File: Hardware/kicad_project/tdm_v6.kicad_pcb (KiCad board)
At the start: 4 copper layers, 65 x 100 mm, 139 parts, among them J1 line_in, J2 headphone_out, J3 battery, J4 DebugHeader, Q1 DMG2305UX-13, SW1 spst_4_pin_internal, SW10 spst_4_pin_internal, SW11 spst_4_pin_internal, SW12 spst_4_pin_internal, SW13 spst_4_pin_internal, SW14 spst_4_pin_internal, SW15 spst_4_pin_internal, SW16 spst_4_pin_internal, SW17 spst_4_pin_internal, SW18 spst_4_pin_internal, SW19 spst_4_pin_internal, SW2 spst_4_pin_internal, SW20 spst_4_pin_internal, SW21 spst_4_pin_internal, SW22 spst_4_pin_internal, SW23 spst_4_pin_internal, SW24 spst_4_pin_internal, SW25 spst_4_pin_internal, SW26 spst_4_pin_internal, SW3 spst_4_pin_internal, SW4 spst_4_pin_internal, SW5 spst_4_pin_internal, SW6 spst_4_pin_internal, SW7 spst_4_pin_internal, SW8 spst_4_pin_internal, SW9 spst_4_pin_internal, U2 Pico, U3 TLV320AIC3204, U4 SPWmicrophone, U5 MCP73831T-2ATI_OT

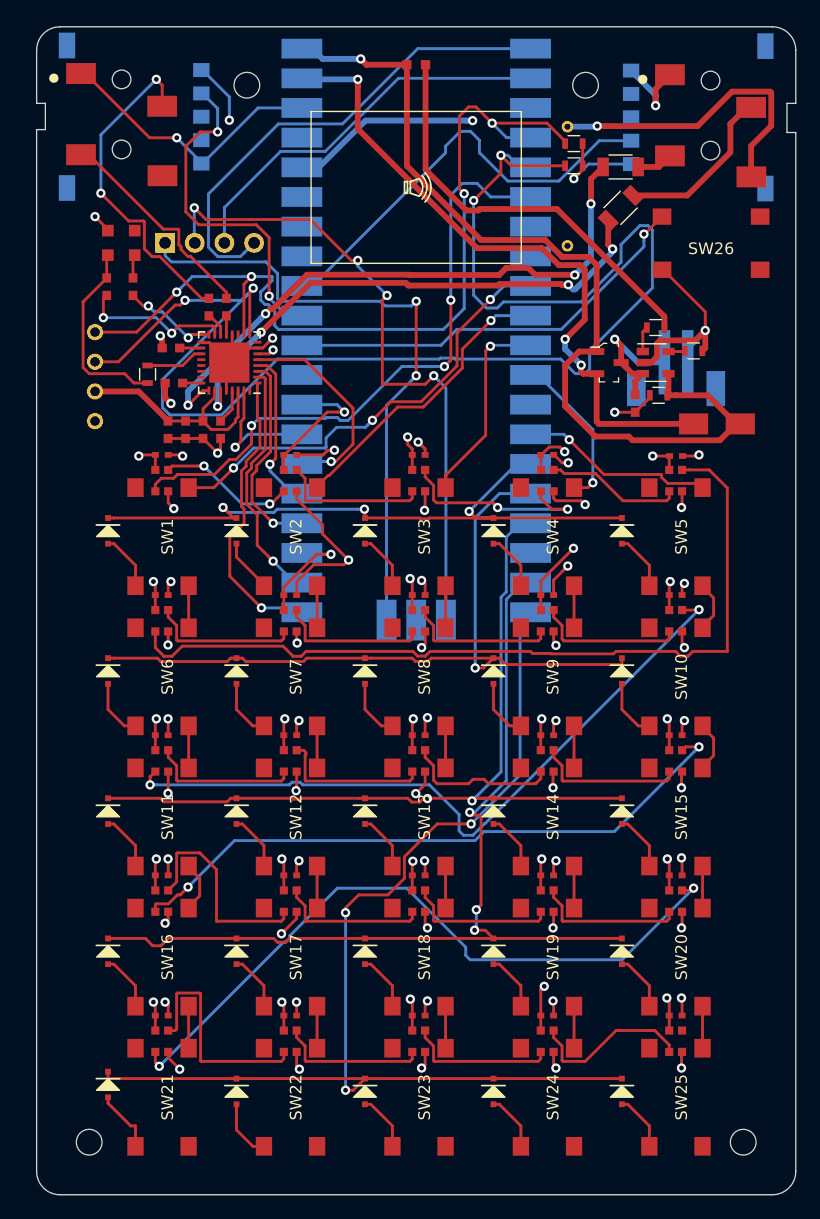
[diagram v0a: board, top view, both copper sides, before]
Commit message: update project with corrected schematic / pcb
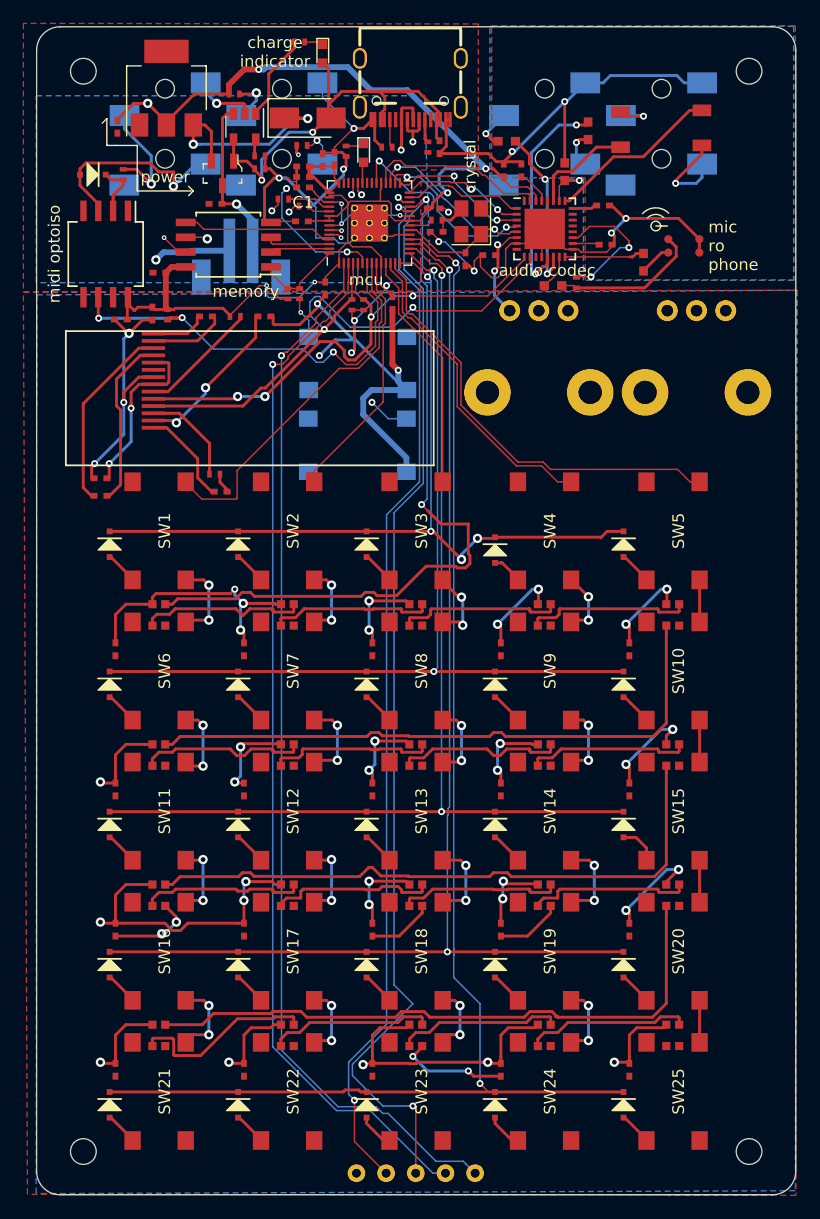
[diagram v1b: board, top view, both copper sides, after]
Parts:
- removed C2, C3, C4, C5: 1u, RandomJunk:C_0402_NoSilk
- removed D1, D2, D3, D4, D5: D, RandomJunk:D_SOD-323F_less_silk
- removed LS1: Speaker, RandomJunk:CMS-181325
- removed OL1: OLED, kbd:OLED_v2
- added C39: .47u, RandomJunk:C_0603_nosilk, F.Cu at (80.5, 40.8)
- added C40: .1uF, RandomJunk:C_0603_nosilk, F.Cu at (78.5, 44.2)
- added C41: 1u, RandomJunk:C_0402_NoSilk, F.Cu at (72.0, 51.4)
- added C42: 10u, RandomJunk:C_0402_NoSilk, F.Cu at (73.3, 44.1)
- added C43: 10u, RandomJunk:C_0402_NoSilk, F.Cu at (81.8, 47.1)
- added C44: .47u, RandomJunk:C_0603_nosilk, F.Cu at (73.5, 41.6)
- added C45: .47u, RandomJunk:C_0603_nosilk, F.Cu at (77.5, 54.0)
- added C46: 10u, RandomJunk:C_0402_NoSilk, F.Cu at (82.0, 50.5)
- added C47: .47u, RandomJunk:C_0603_nosilk, F.Cu at (85.2, 52.0)
- added C48: 47uf, Capacitors_SMD:C_1206, F.Cu at (83.3, 40.6)
- added C49: 47uf, Capacitors_SMD:C_1206, F.Cu at (90.2, 40.5)
- added C50: 10u, RandomJunk:C_0402_NoSilk, F.Cu at (40.5, 56.9)
- added C51: 1u, RandomJunk:C_0402_NoSilk, F.Cu at (47.8, 56.6)
- added C52: 1u, RandomJunk:C_0402_NoSilk, F.Cu at (38.8, 72.0)
- added C53: 1u, RandomJunk:C_0402_NoSilk, F.Cu at (38.8, 70.5)
- added C54: 1u, RandomJunk:C_0402_NoSilk, F.Cu at (43.2, 56.4)
- added C55: 10u, RandomJunk:C_0402_NoSilk, F.Cu at (52.8, 56.6)
- added C56: 10u, RandomJunk:C_0402_NoSilk, F.Cu at (49.0, 71.6)
- added C57: 10u, RandomJunk:C_0402_NoSilk, F.Cu at (48.6, 47.0)
- added C58: 10u, RandomJunk:C_0402_NoSilk, F.Cu at (40.2, 40.4)
- added D53: D_Schottky, Diodes_SMD:D_SMA, F.Cu at (56.5, 39.6)
- added D54: LED, LEDs:LED_0603, F.Cu at (57.8, 34.1)
- added J5: midi_in, RandomJunk:HRO-PJ-327C-A, B.Cu at (44.3, 40.6)
- added J6: midi_out, RandomJunk:HRO-PJ-327C-A, B.Cu at (54.3, 40.6)
- added J7: battery, Connectors_JST:JST_PH_B2B-PH-SM4-TB_02x2.00mm_Straight, B.Cu at (50.8, 52.1)
- added LCD1: 128x32OLED, RandomJunk:oled_ssd1306_14pin_91, F.Cu at (43.3, 62.1)
- added R10: 220, RandomJunk:R_0402_NoSilk, F.Cu at (40.7, 44.5)
- added R11: 1k, RandomJunk:R_0402_NoSilk, F.Cu at (44.5, 56.5)
- added R12: 220, RandomJunk:R_0402_NoSilk, F.Cu at (50.2, 37.6)
- added R13: 220, RandomJunk:R_0402_NoSilk, F.Cu at (56.0, 42.0)
- added R14: 10k, RandomJunk:R_0402_NoSilk, F.Cu at (50.3, 56.6)
- added R15: 330k, RandomJunk:R_0402_NoSilk, F.Cu at (48.5, 70.1)
- added R16: 4.7k, RandomJunk:R_0402_NoSilk, F.Cu at (52.4, 42.9)
- added R17: 1k, RandomJunk:R_0402_NoSilk, F.Cu at (55.8, 33.1)
- added R18: 100k, RandomJunk:R_0402_NoSilk, F.Cu at (52.4, 44.0)
- added R19: 5.1k, RandomJunk:R_0402_NoSilk, F.Cu at (66.8, 42.1)
- added R20: 5.1k, RandomJunk:R_0402_NoSilk, F.Cu at (63.3, 42.1)
- added R7: 1k, RandomJunk:R_0402_NoSilk, F.Cu at (67.5, 48.4)
- added R8: 1k, RandomJunk:R_0402_NoSilk, F.Cu at (59.8, 42.5)
- added R9: 4.7k, RandomJunk:R_0402_NoSilk, F.Cu at (79.5, 53.8)
- added SW27: spst_4_pin_internal, RandomJunk:ts1102_smallerpads_buttonhole, B.Cu at (60.8, 67.6)
- added U1: W25Q32JVSS, Housings_SOIC:SOIJ-8_5.3x5.3mm_Pitch1.27mm, F.Cu at (49.7, 50.5)
- added U6: MCP73831T-2ATI_OT, TO_SOT_Packages_SMD:SOT-23-5, F.Cu at (51.1, 40.4)
- added U7: AMS1117-3.3, TO_SOT_Packages_SMD:SOT-223, F.Cu at (44.4, 37.1)
- added Y1: Crystal_GND24, Crystals:Crystal_SMD_3225-4pin_3.2x2.5mm, F.Cu at (70.5, 48.5)
- C1: footprint RandomJunk:C_0402_NoSilk -> Capacitors_SMD:C_0402_NoSilk
- C26, C30, C31, C34: value 10u -> 100n; footprint RandomJunk:C_0603_nosilk -> RandomJunk:C_0402_NoSilk
- C27, C32: value .47u -> 100n; footprint RandomJunk:C_0603_nosilk -> RandomJunk:C_0402_NoSilk
- C28: value .1uF -> 100n; footprint RandomJunk:C_0603_nosilk -> RandomJunk:C_0402_NoSilk
- C29: value 1.0u -> 100n; footprint RandomJunk:C_0603_nosilk -> RandomJunk:C_0402_NoSilk
- C33: value .47u -> 1u; footprint RandomJunk:C_0603_nosilk -> RandomJunk:C_0402_NoSilk
- C35: value .47u -> 30p; footprint RandomJunk:C_0603_nosilk -> RandomJunk:C_0402_NoSilk
- C36: value 47uf -> 10u; footprint Capacitors_SMD:C_1206 -> RandomJunk:C_0402_NoSilk
- C37: value 47uf -> 30p; footprint Capacitors_SMD:C_1206 -> RandomJunk:C_0402_NoSilk
- C38: footprint RandomJunk:C_0603_nosilk -> RandomJunk:C_0402_NoSilk
- D10, D11, D12, D13, D14, D15, D16, D17, D18, D19, D20, D21, D22, D23, D24, D25, D6, D7, D8, D9: value D -> WS2812B; footprint RandomJunk:D_SOD-323F_less_silk -> RandomJunk:ws2812b-2020-lightpipe
- D26, D27, D28, D29, D30, D31, D32, D33, D34, D35, D36, D37, D38, D39, D40, D41, D42, D43, D44, D45, D46, D47, D48, D49, D50: value WS2812B -> D; footprint RandomJunk:ws2812b-2020-lightpipe -> RandomJunk:D_SOD-323F_less_silk
- D51: value D_Schottky -> LED; footprint Diodes_SMD:D_SMA -> LEDs:LED_0603
- D52: value LED -> D; footprint LEDs:LED_0603 -> RandomJunk:D_SOD-323F_less_silk
- J1: value line_in -> picoprobe_debug; footprint RandomJunk:HRO-PJ-327C-A -> RandomJunk:pico debug header; moved to B.Cu
- J2: value headphone_out -> USB_C_Receptacle_USB2.0; footprint RandomJunk:HRO-PJ-327C-A -> RandomJunk:USB-C_SMD-TYPE-C-31-M-12
- J3: value battery -> line_in; footprint Connectors_JST:JST_PH_B2B-PH-SM4-TB_02x2.00mm_Straight -> RandomJunk:HRO-PJ-327C-A
- J4: value DebugHeader -> headphone_out; footprint Connector_PinSocket_2.54mm:PinSocket_1x04_P2.54mm_Vertical -> RandomJunk:HRO-PJ-327C-A
- R1, R2: value 4.7k -> 27.4; footprint Resistors_SMD:R_0603 -> RandomJunk:R_0402_NoSilk
- R3: value 4.7k -> DNF; footprint Resistors_SMD:R_0603 -> RandomJunk:R_0402_NoSilk
- R4: footprint Resistors_SMD:R_0603 -> RandomJunk:R_0402_NoSilk
- R5: value 1k -> 4.7k; footprint Resistors_SMD:R_0603 -> RandomJunk:R_0402_NoSilk
- R6: value 100k -> 1k; footprint Resistors_SMD:R_0603 -> RandomJunk:R_0402_NoSilk
- RV1, RV2: footprint RandomJunk:rk10j -> Potentiometers:Potentiometer_Alps_RK09K_Horizontal; moved to F.Cu
- SW26: moved to B.Cu
- U2: value Pico -> RP2040; footprint RandomJunk:RPi_Pico_SMD_only -> MCU_RaspberryPi_and_Boards:RP2040-QFN-56; moved to F.Cu
- U4: value SPWmicrophone -> AP3722AT_mic; footprint RandomJunk:SPW2430HR5H-B -> RandomJunk:AP3722AT-SMD-mic
- U5: value MCP73831T-2ATI_OT -> 6N137; footprint TO_SOT_Packages_SMD:SOT-23-5 -> Housings_SOIC:SO-8_5.3x6.2mm_Pitch1.27mm
- moved J1 93.6 mm to (65.8, 130.0), turned to 0 degrees
- moved H1 92.4 mm to (37.3, 128.1)
- moved H3 92.4 mm to (94.3, 128.1)
- moved H2 91.7 mm to (37.3, 35.6)
- moved H4 91.7 mm to (94.3, 35.6)
- moved U4 48.2 mm to (88.7, 50.6), turned to 90 degrees
- moved U5 48.0 mm to (39.2, 51.3), turned to 270 degrees
- moved J4 43.6 mm to (86.8, 40.6)
- moved RV1 39.1 mm to (73.8, 56.1)
- moved D51 38.1 mm to (61.3, 42.6), turned to 270 degrees
- moved Q1 36.8 mm to (49.2, 44.4), turned to 270 degrees
- moved SW26 32.0 mm to (60.8, 60.6), turned to 180 degrees
- moved R6 31.9 mm to (55.8, 54.7), turned to 270 degrees
- moved R4 29.5 mm to (60.3, 55.6), turned to 90 degrees
- moved U3 29.3 mm to (76.8, 49.1), turned to 0 degrees
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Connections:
- C1 pad 1: +3V3 -> Net-(C1-Pad1)
- C26 pad 1: GND -> +3V3
- C26 pad 2: Net-(C26-Pad2) -> GND
- C27 pad 1: Net-(C27-Pad1) -> +3V3
- C27 pad 2: Net-(C27-Pad2) -> GND
- C31 pad 1: Net-(C31-Pad1) -> +3V3
- C32 pad 1: Net-(C32-Pad1) -> +3V3
- C32 pad 2: Net-(C32-Pad2) -> GND
- C33 pad 1: Net-(C33-Pad1) -> +3V3
- C33 pad 2: Net-(C33-Pad2) -> GND
- C34 pad 1: GND -> +3V3
- C34 pad 2: Net-(C34-Pad2) -> GND
- C35 pad 1: Net-(C35-Pad1) -> /XIN
- C35 pad 2: Net-(C35-Pad2) -> GND
- C36 pad 1: Net-(C36-Pad1) -> VBUS
- C36 pad 2: Net-(C36-Pad2) -> GND
- C37 pad 2: Net-(C37-Pad2) -> GND
- C38 pad 1: +BATT -> GND
- C38 pad 2: GND -> Net-(C38-Pad2)
- D10 pad 1: key_row2 -> Net-(D10-Pad1)
- D10 pad 2: Net-(D10-Pad2) -> GND
- D11 pad 1: key_row3 -> Net-(D11-Pad1)
- D11 pad 2: Net-(D11-Pad2) -> GND
- D12 pad 1: key_row3 -> Net-(D12-Pad1)
- D12 pad 2: Net-(D12-Pad2) -> GND
- D13 pad 1: key_row3 -> Net-(D13-Pad1)
- D13 pad 2: Net-(D13-Pad2) -> GND
- D14 pad 1: key_row3 -> Net-(D14-Pad1)
- D14 pad 2: Net-(D14-Pad2) -> GND
- D15 pad 1: key_row3 -> Net-(D15-Pad1)
- D15 pad 2: Net-(D15-Pad2) -> GND
- D16 pad 1: key_row4 -> Net-(D16-Pad1)
- D16 pad 2: Net-(D16-Pad2) -> GND
- D17 pad 1: key_row4 -> Net-(D17-Pad1)
- D17 pad 2: Net-(D17-Pad2) -> GND
- D18 pad 1: key_row4 -> Net-(D18-Pad1)
- D18 pad 2: Net-(D18-Pad2) -> GND
- D19 pad 1: key_row4 -> Net-(D19-Pad1)
- D19 pad 2: Net-(D19-Pad2) -> GND
- D20 pad 1: key_row4 -> Net-(D20-Pad1)
- D20 pad 2: Net-(D20-Pad2) -> GND
- D21 pad 1: key_row5 -> Net-(D21-Pad1)
- D21 pad 2: Net-(D21-Pad2) -> GND
- D22 pad 1: key_row5 -> Net-(D22-Pad1)
- D22 pad 2: Net-(D22-Pad2) -> GND
- D23 pad 1: key_row5 -> Net-(D23-Pad1)
- D23 pad 2: Net-(D23-Pad2) -> GND
- D24 pad 1: key_row5 -> Net-(D24-Pad1)
- D24 pad 2: Net-(D24-Pad2) -> GND
- D25 pad 1: key_row5 -> Net-(D25-Pad1)
- D25 pad 2: Net-(D25-Pad2) -> GND
- D26 pad 1: Net-(D26-Pad1) -> key_row1
- D26 pad 2: GND -> Net-(D26-Pad2)
- D27 pad 1: Net-(D27-Pad1) -> key_row1
- D27 pad 2: GND -> Net-(D27-Pad2)
- D28 pad 1: Net-(D28-Pad1) -> key_row1
- D28 pad 2: GND -> Net-(D28-Pad2)
- D29 pad 1: Net-(D29-Pad1) -> key_row1
- D29 pad 2: GND -> Net-(D29-Pad2)
- D30 pad 1: Net-(D30-Pad1) -> key_row1
- D30 pad 2: GND -> Net-(D30-Pad2)
- D31 pad 1: Net-(D31-Pad1) -> key_row2
- D31 pad 2: GND -> Net-(D31-Pad2)
- D32 pad 1: Net-(D32-Pad1) -> key_row2
- D32 pad 2: GND -> Net-(D32-Pad2)
- D33 pad 1: Net-(D33-Pad1) -> key_row2
- D33 pad 2: GND -> Net-(D33-Pad2)
- D34 pad 1: Net-(D34-Pad1) -> key_row2
- D34 pad 2: GND -> Net-(D34-Pad2)
- D35 pad 1: Net-(D35-Pad1) -> key_row2
- D35 pad 2: GND -> Net-(D35-Pad2)
- D36 pad 1: Net-(D36-Pad1) -> key_row3
- D36 pad 2: GND -> Net-(D36-Pad2)
- D37 pad 1: Net-(D37-Pad1) -> key_row3
- D37 pad 2: GND -> Net-(D37-Pad2)
- D38 pad 1: Net-(D38-Pad1) -> key_row3
- D38 pad 2: GND -> Net-(D38-Pad2)
- D39 pad 1: Net-(D39-Pad1) -> key_row3
- D39 pad 2: GND -> Net-(D39-Pad2)
- D40 pad 1: Net-(D40-Pad1) -> key_row3
- D40 pad 2: GND -> Net-(D40-Pad2)
- D41 pad 1: Net-(D41-Pad1) -> key_row4
- D41 pad 2: GND -> Net-(D41-Pad2)
- D42 pad 1: Net-(D42-Pad1) -> key_row4
- D42 pad 2: GND -> Net-(D42-Pad2)
- D43 pad 1: Net-(D43-Pad1) -> key_row4
- D43 pad 2: GND -> Net-(D43-Pad2)
- D44 pad 1: Net-(D44-Pad1) -> key_row4
- D44 pad 2: GND -> Net-(D44-Pad2)
- D45 pad 1: Net-(D45-Pad1) -> key_row4
- D45 pad 2: GND -> Net-(D45-Pad2)
- D46 pad 1: Net-(D46-Pad1) -> key_row5
- D46 pad 2: GND -> Net-(D46-Pad2)
- D47 pad 1: Net-(D47-Pad1) -> key_row5
- D47 pad 2: GND -> Net-(D47-Pad2)
- D48 pad 1: Net-(D48-Pad1) -> key_row5
- D48 pad 2: GND -> Net-(D48-Pad2)
- D49 pad 1: Net-(D49-Pad1) -> key_row5
- D49 pad 2: GND -> Net-(D49-Pad2)
- D50 pad 1: (no net) -> key_row5
- D50 pad 2: GND -> Net-(D50-Pad2)
- D51 pad 1: vsys -> Net-(D51-Pad1)
- D51 pad 2: VBUS -> Net-(D51-Pad2)
- D52 pad 2: VBUS -> Net-(D52-Pad2)
- D6 pad 1: key_row2 -> Net-(D6-Pad1)
- D6 pad 2: Net-(D6-Pad2) -> GND
- D7 pad 1: key_row2 -> Net-(D7-Pad1)
- D7 pad 2: Net-(D7-Pad2) -> GND
- D8 pad 1: key_row2 -> Net-(D8-Pad1)
- D8 pad 2: Net-(D8-Pad2) -> GND
- D9 pad 1: key_row2 -> Net-(D10-Pad3)
- D9 pad 2: Net-(D9-Pad2) -> GND
- J1 pad 2: Net-(C27-Pad2) -> swclk
- J1 pad 3: Net-(C32-Pad2) -> swdio
- J1 pad 4: (no net) -> rx
- J3 pad 1: +BATT -> GND
- J3 pad 2: GND -> Net-(C39-Pad2)
- J4 pad 1: Net-(J4-Pad1) -> GND
- J4 pad 2: Net-(J4-Pad2) -> Net-(C49-Pad1)
- J4 pad 3: Net-(J4-Pad3) -> Net-(C48-Pad1)
- Q1 pad 2: vsys -> Net-(D53-Pad1)
- R1 pad 1: +3V3 -> Net-(R1-Pad1)
- R1 pad 2: sda -> /USB_D+
- R2 pad 1: +3V3 -> Net-(R2-Pad1)
- R2 pad 2: scl -> /USB_D-
- R3 pad 1: Net-(C33-Pad2) -> +3V3
- R3 pad 2: Net-(R3-Pad2) -> /QSPI_SS
- R4 pad 1: Net-(R4-Pad1) -> +3V3
- R4 pad 2: GND -> sda
- R5 pad 1: Net-(D52-Pad1) -> +3V3
- R5 pad 2: Net-(R5-Pad2) -> scl
- R6 pad 1: GND -> /QSPI_SS
- R6 pad 2: VBUS -> Net-(R6-Pad2)
- SW1 pad 1: Net-(D1-Pad2) -> Net-(D26-Pad2)
- SW1 pad 2: (no net) -> Net-(SW1-Pad2)
- SW10 pad 1: Net-(D10-Pad2) -> Net-(D35-Pad2)
- SW10 pad 2: (no net) -> Net-(SW10-Pad2)
- SW11 pad 1: Net-(D11-Pad2) -> Net-(D36-Pad2)
- SW11 pad 2: (no net) -> Net-(SW11-Pad2)
- SW12 pad 1: Net-(D12-Pad2) -> Net-(D37-Pad2)
- SW12 pad 2: (no net) -> Net-(SW12-Pad2)
- SW13 pad 1: Net-(D13-Pad2) -> Net-(D38-Pad2)
- SW13 pad 2: (no net) -> Net-(SW13-Pad2)
- SW14 pad 1: Net-(D14-Pad2) -> Net-(D39-Pad2)
- SW14 pad 2: (no net) -> Net-(SW14-Pad2)
- SW15 pad 1: Net-(D15-Pad2) -> Net-(D40-Pad2)
- SW15 pad 2: (no net) -> Net-(SW15-Pad2)
- SW16 pad 1: Net-(D16-Pad2) -> Net-(D41-Pad2)
- SW16 pad 2: (no net) -> Net-(SW16-Pad2)
- SW17 pad 1: Net-(D17-Pad2) -> Net-(D42-Pad2)
- SW17 pad 2: (no net) -> Net-(SW17-Pad2)
- SW18 pad 1: Net-(D18-Pad2) -> Net-(D43-Pad2)
- SW18 pad 2: (no net) -> Net-(SW18-Pad2)
- SW19 pad 1: Net-(D19-Pad2) -> Net-(D44-Pad2)
- SW19 pad 2: (no net) -> Net-(SW19-Pad2)
- SW2 pad 1: Net-(D2-Pad2) -> Net-(D27-Pad2)
- SW2 pad 2: (no net) -> Net-(SW2-Pad2)
- SW20 pad 1: Net-(D20-Pad2) -> Net-(D45-Pad2)
- SW20 pad 2: (no net) -> Net-(SW20-Pad2)
- SW21 pad 1: Net-(D21-Pad2) -> Net-(D46-Pad2)
- SW21 pad 2: (no net) -> Net-(SW21-Pad2)
- SW21 pad 3: (no net) -> Net-(SW21-Pad3)
- SW22 pad 1: Net-(D22-Pad2) -> Net-(D47-Pad2)
- SW22 pad 2: (no net) -> Net-(SW22-Pad2)
- SW22 pad 3: (no net) -> Net-(SW22-Pad3)
- SW23 pad 1: Net-(D23-Pad2) -> Net-(D48-Pad2)
- SW23 pad 2: (no net) -> Net-(SW23-Pad2)
- SW23 pad 3: (no net) -> Net-(SW23-Pad3)
- SW24 pad 1: Net-(D24-Pad2) -> Net-(D49-Pad2)
- SW24 pad 2: (no net) -> Net-(SW24-Pad2)
- SW24 pad 3: (no net) -> Net-(SW24-Pad3)
- SW25 pad 1: Net-(D25-Pad2) -> Net-(D50-Pad2)
- SW25 pad 2: (no net) -> Net-(SW25-Pad2)
- SW25 pad 3: (no net) -> Net-(SW25-Pad3)
- SW26 pad 2: (no net) -> Net-(R6-Pad2)
- SW26 pad 4: (no net) -> Net-(SW26-Pad4)
- SW3 pad 1: Net-(D3-Pad2) -> Net-(D28-Pad2)
- SW3 pad 2: (no net) -> Net-(SW3-Pad2)
- SW4 pad 1: Net-(D4-Pad2) -> Net-(D29-Pad2)
- SW4 pad 2: (no net) -> Net-(SW4-Pad2)
- SW5 pad 1: Net-(D5-Pad2) -> Net-(D30-Pad2)
- SW5 pad 2: (no net) -> Net-(SW5-Pad2)
- SW6 pad 1: Net-(D6-Pad2) -> Net-(D31-Pad2)
- SW6 pad 2: (no net) -> Net-(SW6-Pad2)
- SW7 pad 1: Net-(D7-Pad2) -> Net-(D32-Pad2)
- SW7 pad 2: (no net) -> Net-(SW7-Pad2)
- SW8 pad 1: Net-(D8-Pad2) -> Net-(D33-Pad2)
- SW8 pad 2: (no net) -> Net-(SW8-Pad2)
- SW9 pad 1: Net-(D9-Pad2) -> Net-(D34-Pad2)
- SW9 pad 2: (no net) -> Net-(SW9-Pad2)
- U2 pad 1: Net-(J4-Pad4) -> +3V3
- U2 pad 10: key_col2 -> +3V3
- U2 pad 13: (no net) -> key_col5
- U2 pad 14: key_col5 -> key_row1
- U2 pad 15: key_row1 -> key_row2
- U2 pad 16: key_row2 -> key_row3
- U2 pad 17: key_row3 -> key_row4
- U2 pad 18: (no net) -> key_row5
- U2 pad 19: key_row4 -> GND
- U2 pad 2: Net-(J4-Pad3) -> tx
- U2 pad 20: key_row5 -> /XIN
- U2 pad 21: mclk -> /XOUT
- U2 pad 22: bck -> +3V3
- U2 pad 23: GND -> Net-(C1-Pad1)
- U2 pad 24: lrclk -> swclk
- U2 pad 25: din -> swdio
- U2 pad 26: dout -> Net-(SW27-Pad1)
- U2 pad 27: codec_reset -> mclk
- U2 pad 28: GND -> bck
- U2 pad 29: (no net) -> lrclk
- U2 pad 3: (no net) -> rx
- U2 pad 30: Net-(SW26-Pad1) -> din
- U2 pad 31: pot1 -> dout
- U2 pad 32: pot2 -> codec_reset
- U2 pad 33: (no net) -> +3V3
- U2 pad 34: (no net) -> led_din
- U2 pad 35: (no net) -> Net-(U2-Pad35)
- U2 pad 36: +3V3 -> Net-(U2-Pad36)
- U2 pad 37: (no net) -> Net-(D51-Pad2)
- U2 pad 38: GND -> pot1
- U2 pad 39: vsys -> pot2
- U2 pad 40: VBUS -> Net-(U2-Pad40)
- U2 pad 41: Net-(J4-Pad2) -> Net-(U2-Pad41)
- U2 pad 42: (no net) -> +3V3
- U2 pad 43: Net-(J4-Pad1) -> +3V3
- U2 pad 6: led_din -> /MIDI_TX
- U2 pad 7: (no net) -> /MIDI_RX
- U2 pad 8: (no net) -> key_col1
- U2 pad 9: key_col1 -> key_col2
- U3 pad 11: (no net) -> Net-(U3-Pad11)
- U3 pad 13: Net-(C27-Pad1) -> Net-(C39-Pad1)
- U3 pad 14: Net-(C32-Pad1) -> Net-(C44-Pad1)
- U3 pad 15: Net-(C33-Pad1) -> Net-(C45-Pad1)
- U3 pad 16: Net-(C35-Pad1) -> Net-(C47-Pad1)
- U3 pad 18: Net-(C34-Pad2) -> Net-(C46-Pad2)
- U3 pad 19: Net-(R3-Pad2) -> Net-(R9-Pad2)
- U3 pad 20: (no net) -> Net-(U3-Pad20)
- U3 pad 21: (no net) -> Net-(U3-Pad21)
- U3 pad 22: (no net) -> Net-(U3-Pad22)
- U3 pad 23: (no net) -> Net-(U3-Pad23)
- U3 pad 24: Net-(C31-Pad1) -> Net-(C43-Pad1)
- U3 pad 25: Net-(C37-Pad2) -> Net-(C49-Pad2)
- U3 pad 27: Net-(C36-Pad2) -> Net-(C48-Pad2)
- U3 pad 29: Net-(C26-Pad2) -> Net-(C38-Pad2)
- U3 pad 32: (no net) -> Net-(U3-Pad32)
- U3 pad 8: (no net) -> Net-(U3-Pad8)
- U4 pad 1: GND -> Net-(C45-Pad2)
- U4 pad 2: Net-(C33-Pad2) -> GND
- U4 pad 3: Net-(C35-Pad2) -> GND
- U4 pad 4: (no net) -> Net-(C47-Pad2)
- U5 pad 1: Net-(R5-Pad2) -> Net-(U5-Pad1)
- U5 pad 2: GND -> Net-(D52-Pad1)
- U5 pad 3: +BATT -> Net-(D52-Pad2)
- U5 pad 4: VBUS -> Net-(U5-Pad4)
- U5 pad 5: Net-(R4-Pad1) -> GND
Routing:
- net +3V3: track 140.2 -> 354.0 mm, vias 53 -> 46
- net swdio: track 0.00 -> 94.1 mm, vias 0 -> 2
- net tx: track 0.00 -> 90.6 mm, vias 0 -> 1
- net rx: track 0.00 -> 89.7 mm, vias 0 -> 1
- net swclk: track 0.00 -> 89.1 mm, vias 0 -> 2
- net scl: track 127.5 -> 45.2 mm
- net Net-(D30-Pad1): track 70.9 -> 0.00 mm
- net GND: track 167.6 -> 238.4 mm, vias 34 -> 22
- net Net-(D35-Pad1): track 60.6 -> 0.00 mm, vias 2 -> 0
- net Net-(D45-Pad1): track 60.1 -> 0.00 mm, vias 2 -> 0
- net vsys: track 56.5 -> 0.00 mm, vias 3 -> 0
- net Net-(J4-Pad2): track 55.8 -> 0.00 mm, vias 4 -> 0
- net Net-(D40-Pad1): track 54.3 -> 0.00 mm, vias 2 -> 0
- net Net-(D20-Pad1): track 0.00 -> 53.3 mm
- net Net-(D15-Pad1): track 0.00 -> 53.3 mm
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- added copper zone on B.Cu, net +3V3
- added copper zone on B.Cu, net GND
- added copper zone on F.Cu, net GND
- added copper zone on In2.Cu, net GND
- removed copper zone on In2.Cu, net +3V3
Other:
- outline, holes or cut-outs redrawn
- rule trace_min: 0.2 -> 0.09
- rule via_min_drill: 0.3 -> 0.2
- board text added: "+"
- board text added: "Audio In"
- board text added: "Audio Out"
- board text added: "RUN"
- board text added: "SAFEBOOT"
- board text added: "audio codec"
- board text added: "battery"
- board text added: "charge indicator"
- board text added: "crystal"
- board text added: "mcu"
- board text added: "memory"
- board text added: "mic ro phone"
- board text added: "midi optoiso"
- board text added: "power"
